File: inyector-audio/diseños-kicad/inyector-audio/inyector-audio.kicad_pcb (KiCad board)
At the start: 2 copper layers, 35 x 34 mm, 7 parts, among them J1 Ent, J2 Sal, U1 NE555

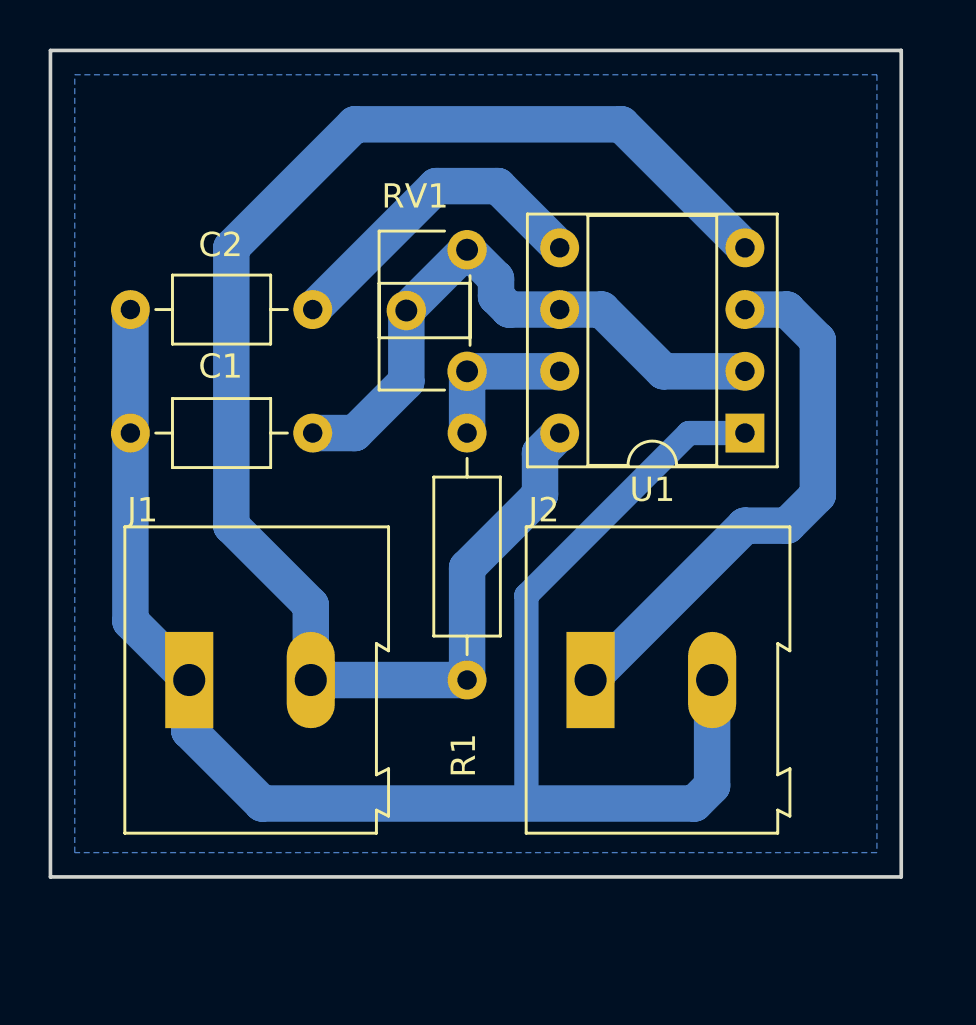
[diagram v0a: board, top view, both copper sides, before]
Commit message: Add files via upload
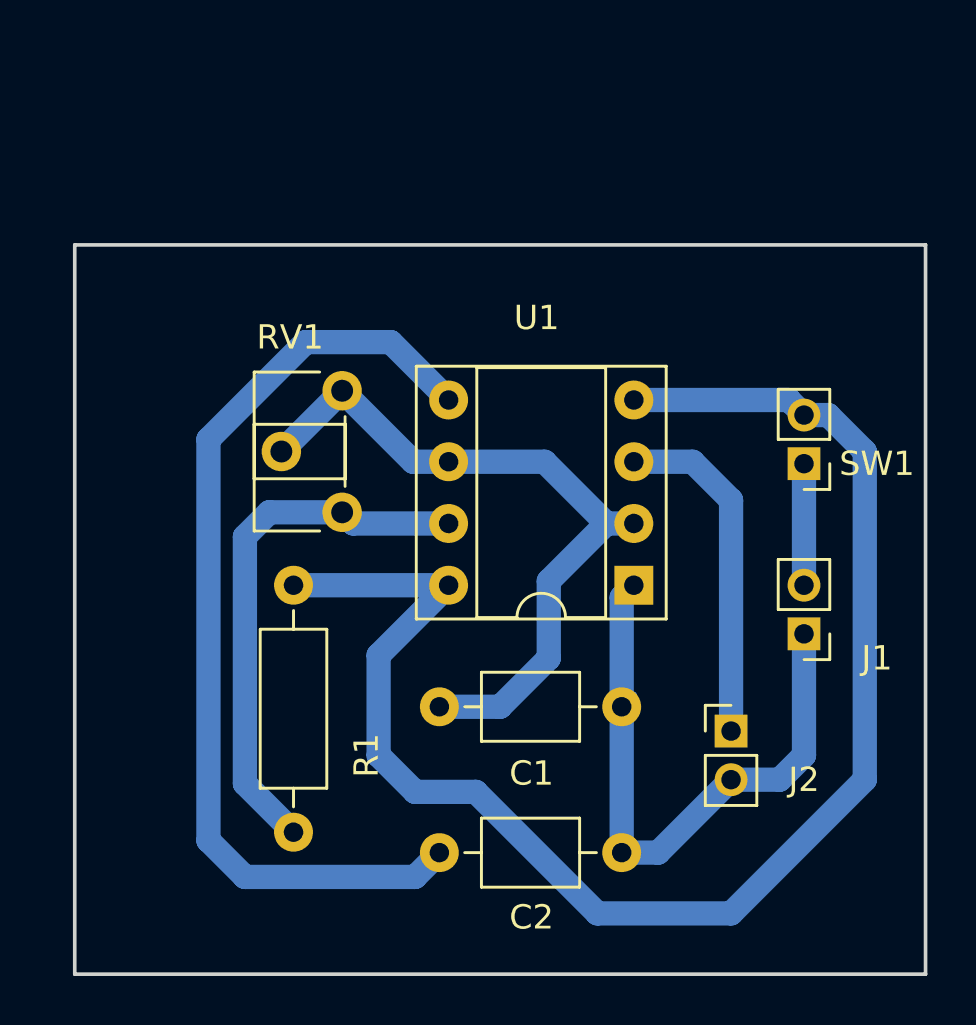
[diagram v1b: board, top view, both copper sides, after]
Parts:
- added SW1: SW_DIP_x01, Connector_PinHeader_2.00mm:PinHeader_1x02_P2.00mm_Vertical, F.Cu at (115.0, 80.0)
- J1, J2: footprint TerminalBlock:TerminalBlock_Altech_AK300-2_P5.00mm -> Connector_PinHeader_2.00mm:PinHeader_1x02_P2.00mm_Vertical
- moved J1 25.4 mm to (115.0, 87.0), turned to 180 degrees
- moved C2 22.9 mm to (100.0, 96.0), turned to 0 degrees
- moved C1 12.4 mm to (100.0, 90.0), turned to 0 degrees
- moved R1 8.14 mm to (94.0, 85.0), turned to 270 degrees
- moved U1 7.75 mm to (108.0, 85.0)
- moved RV1 7.75 mm to (96.0, 82.0)
- moved J2 6.15 mm to (112.0, 91.0)
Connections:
- J1 pad 2: +9V -> Net-(J1-Pad2)
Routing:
- net GND: track 65.5 -> 26.1 mm
- net Net-(C2-Pad1): track 13.3 -> 39.6 mm
- net Net-(R1-Pad2): track 6.35 -> 22.0 mm
- net Net-(J2-Pad1): track 22.4 -> 14.2 mm
- net Net-(J1-Pad2): track 0.00 -> 5.00 mm
- net Net-(C1-Pad1): track 25.1 -> 29.6 mm
- net +9V: track 62.6 -> 63.4 mm
- removed copper zone on B.Cu, net GND
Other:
- board size 35 x 34 mm -> 35 x 30 mm
